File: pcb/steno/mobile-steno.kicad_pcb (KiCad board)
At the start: 2 copper layers, 188 x 92.5 mm, 65 parts, among them J1 Conn_01x02, J2 Conn_01x04, J3 Conn_01x02, K1 KEYSW, K10 KEYSW, K11 KEYSW, K12 KEYSW, K13 KEYSW, K14 KEYSW, K15 KEYSW, K16 KEYSW, K17 KEYSW, K18 KEYSW, K19 KEYSW, K2 KEYSW, K20 KEYSW, K21 KEYSW, K22 KEYSW, K23 KEYSW, K24 KEYSW, K25 KEYSW, K26 KEYSW, K27 KEYSW, K28 KEYSW, K29 KEYSW, K3 KEYSW, K30 KEYSW, K4 KEYSW, K5 KEYSW, K6 KEYSW, K7 KEYSW, K8 KEYSW, K9 KEYSW, U1 Adafruit_Feather, U2 MT25QL128ABA1ESE

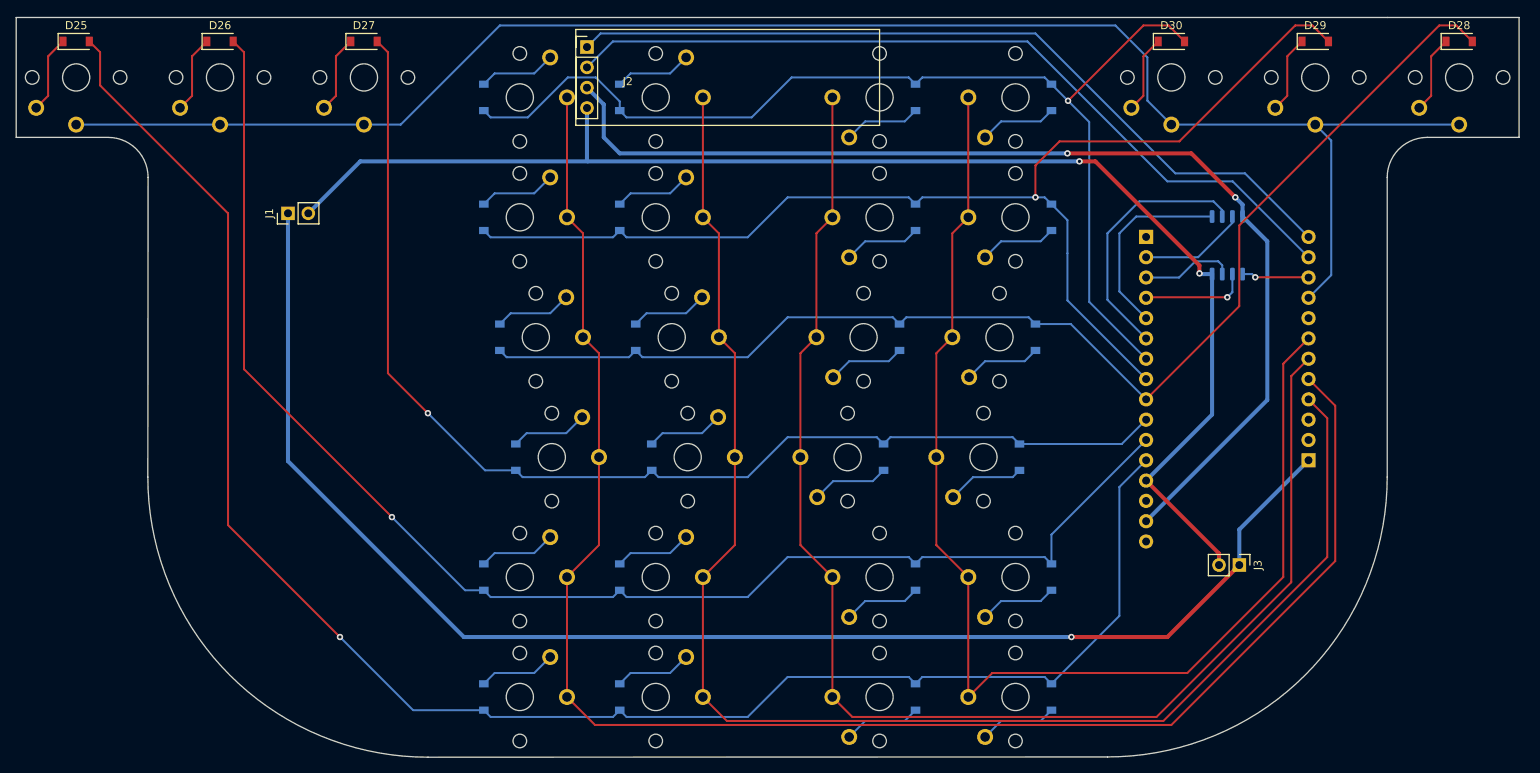
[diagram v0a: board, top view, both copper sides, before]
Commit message: Update PCB
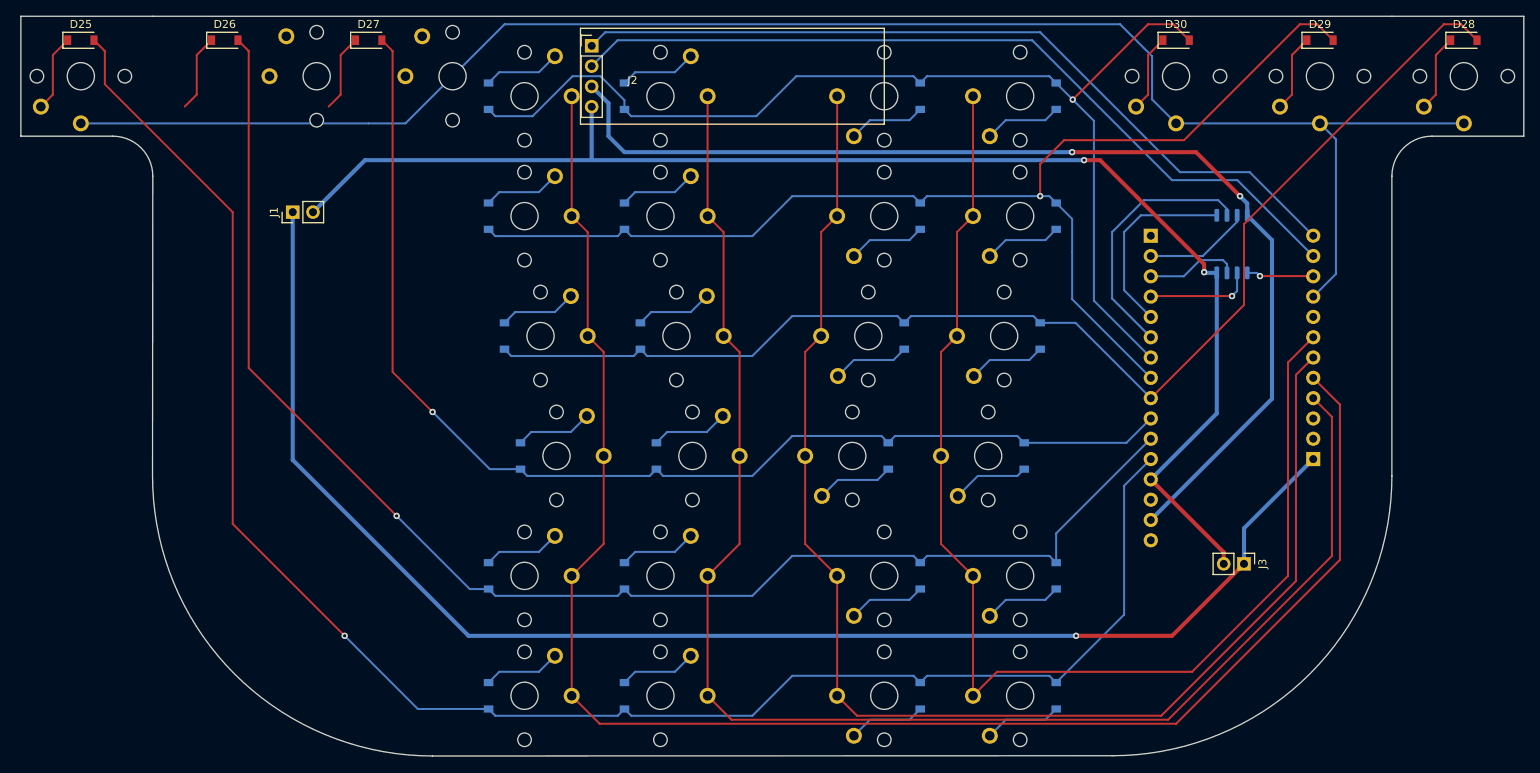
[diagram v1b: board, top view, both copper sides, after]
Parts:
- moved K26 12.1 mm to (59.5, 40.0), turned to 270 degrees
- moved K27 11.1 mm to (76.5, 40.0), turned to 270 degrees
- moved D1 0.61 mm to (98.0, 117.5)
- moved D10 0.61 mm to (83.0, 72.5)
- moved D11 0.61 mm to (81.0, 57.5)
- moved D12 0.61 mm to (81.0, 42.5)
- moved D2 0.61 mm to (98.0, 102.5)
- moved D27 0.61 mm to (66.0, 35.5)
- moved D3 0.61 mm to (102.0, 87.5)
- moved D4 0.61 mm to (100.0, 72.5)
- moved D5 0.61 mm to (98.0, 57.5)
- moved D6 0.61 mm to (98.0, 42.5)
- moved D7 0.61 mm to (81.0, 117.5)
- moved D8 0.61 mm to (81.0, 102.5)
- moved D9 0.61 mm to (85.0, 87.5)
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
